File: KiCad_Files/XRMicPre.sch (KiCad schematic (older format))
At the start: 28 parts

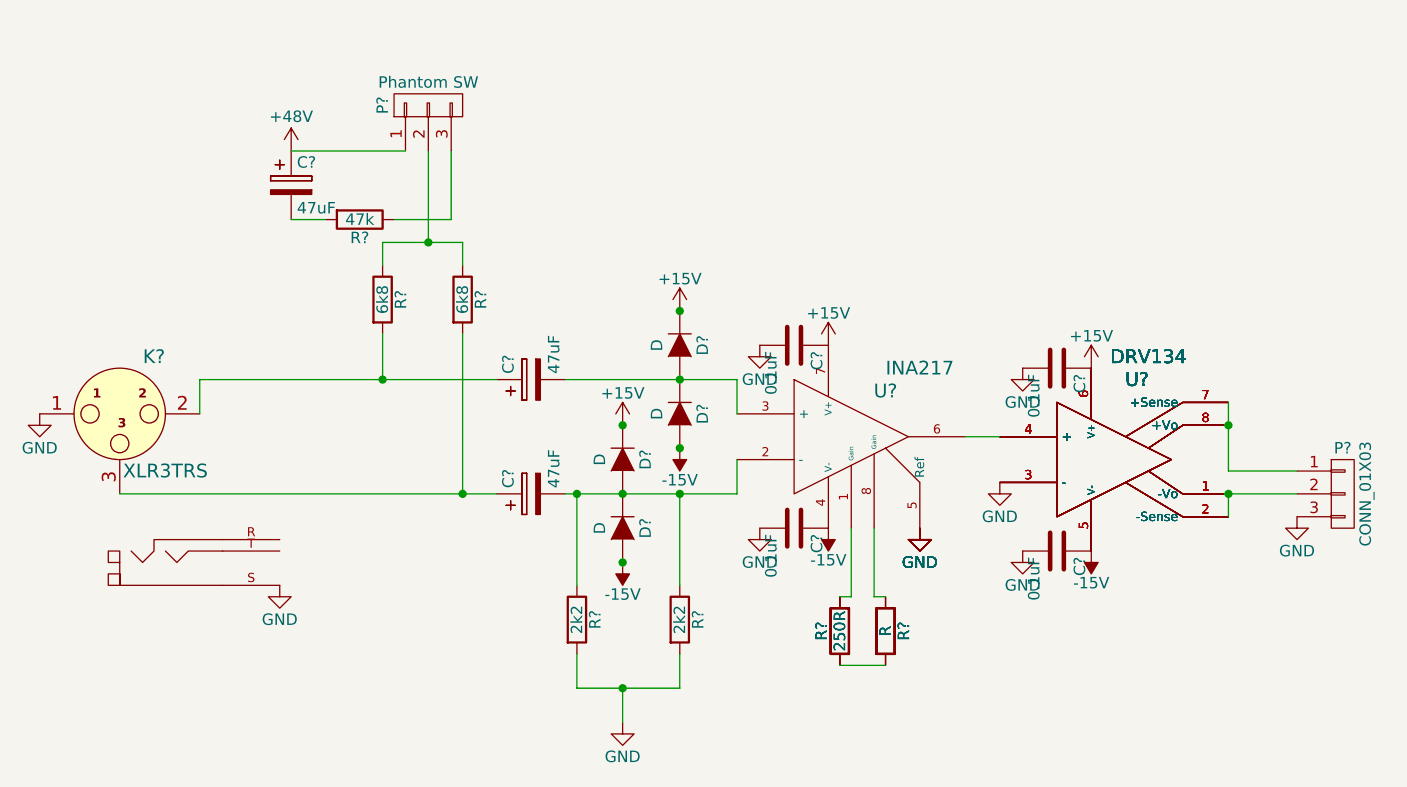
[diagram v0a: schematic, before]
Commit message: Working on PCB
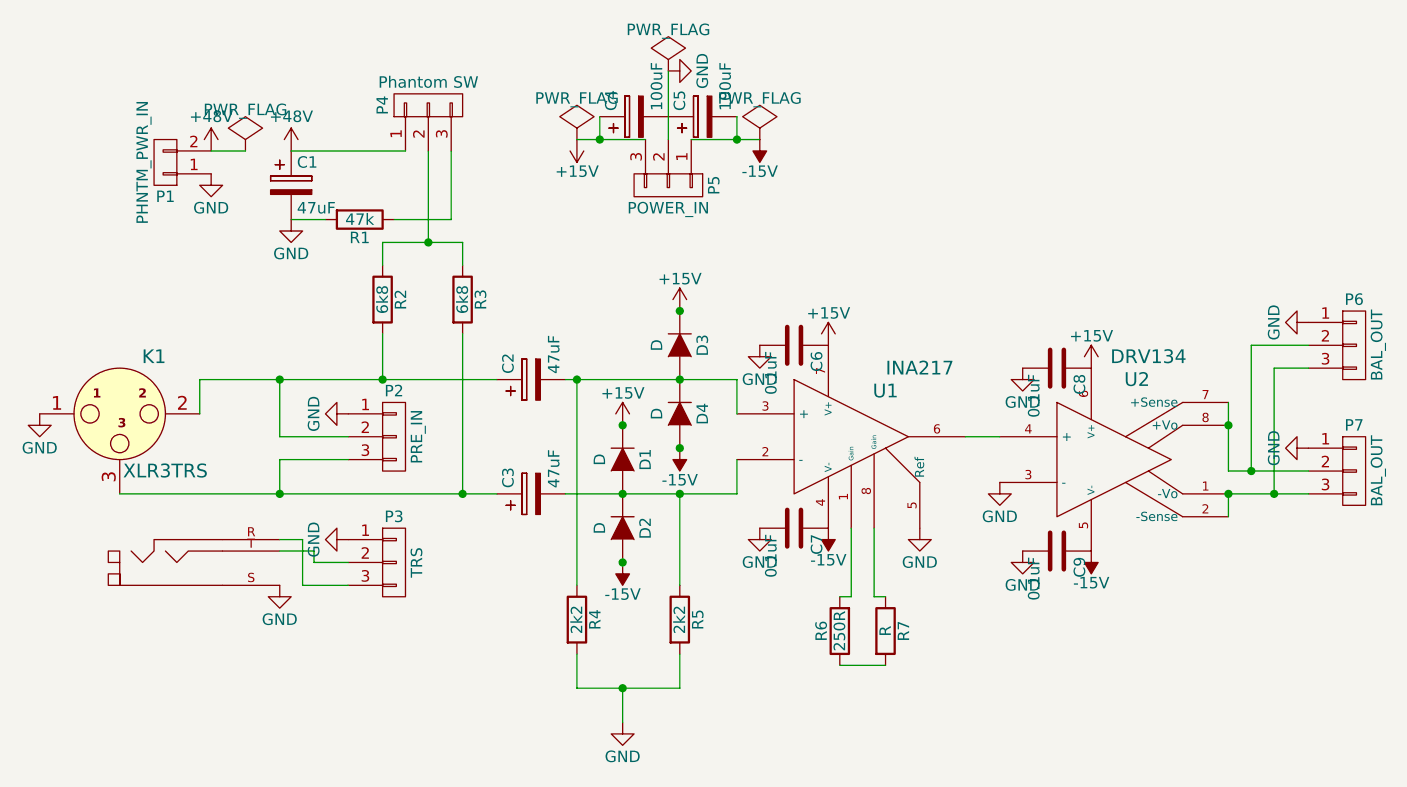
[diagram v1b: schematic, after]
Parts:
- removed R?: 250R, symbol R
- removed R?: R, symbol R
- removed U? (x3): DRV134, symbol DRV134
- added C4, C5: 100uF, Capacitors_ThroughHole:C_Radial_D6.3_L11.2_P2.5, symbol CP
- added P1: PHNTM_PWR_IN, Socket_Strips:Socket_Strip_Straight_1x02, symbol CONN_01X02
- added P2: PRE_IN, Socket_Strips:Socket_Strip_Straight_1x03, symbol CONN_01X03
- added P3: TRS, Socket_Strips:Socket_Strip_Straight_1x03, symbol CONN_01X03
- added P5: POWER_IN, Socket_Strips:Socket_Strip_Straight_1x03, symbol CONN_01X03
- added P6: BAL_OUT, Socket_Strips:Socket_Strip_Straight_1x03, symbol CONN_01X03
- C1, C2, C3: renamed from C?; footprint (none) -> Capacitors_ThroughHole:C_Radial_D6.3_L11.2_P2.5
- C6, C7, C8, C9: renamed from C?; footprint (none) -> Discret:C1-1
- D1, D2, D3, D4: renamed from D?; footprint (none) -> Diodes_SMD:MiniMELF_Standard
- K1: renamed from K?; footprint (none) -> def-footprints:NCJ6FA-V
- P4: renamed from P?; footprint (none) -> Socket_Strips:Socket_Strip_Straight_1x03
- P7: renamed from P?; value CONN_01X03 -> BAL_OUT; footprint (none) -> Socket_Strips:Socket_Strip_Straight_1x03
- R1, R2, R3, R4, R5, R6: renamed from R?; footprint (none) -> Resistors_SMD:R_0805_HandSoldering
- R7: renamed from R?; footprint (none) -> Socket_Strips:Socket_Strip_Straight_1x02
- U1, U2: renamed from U?; footprint (none) -> def-footprints:DIP8+SOIC8_1
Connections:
- net +15V: now also C4.1, P5.3 (P3)
- net +48V: now also P1.2 (P2)
- net -15V: now also C5.2, P5.1 (P1)
- net GND: now also C1.2, P7.1 (P1), R1.2, P1.1 (P1), P2.1 (P1), P3.1 (P1), P5.2 (P2), P6.1 (P1); no longer P7.3 (P3)
- net at C3.2, D1.2 (A), D2.1 (K)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: no longer R4.1
- net at C2.2, D3.2 (A), D4.1 (K)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: now also R4.1
- net at C3.1, K1.3, R3.2: now also P2.3 (P3)
- net at C2.1, K1.2, R2.2: now also P2.2 (P2)
- net at U2.1 (-Vo), U2.2 (-Sense): now also P7.3 (P3), P6.3 (P3); no longer P7.2 (P2)
- net at U2.7 (+Sense), U2.8 (+Vo): now also P7.2 (P2), P6.2 (P2); no longer P7.1 (P1)
- net at K1.R: now also P3.3 (P3)
- net at K1.T: now also P3.2 (P2)
- new net: C4.2, C5.1
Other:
- moved on the sheet: P7
